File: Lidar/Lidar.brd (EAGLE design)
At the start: 100 x 80 mm, 4 parts

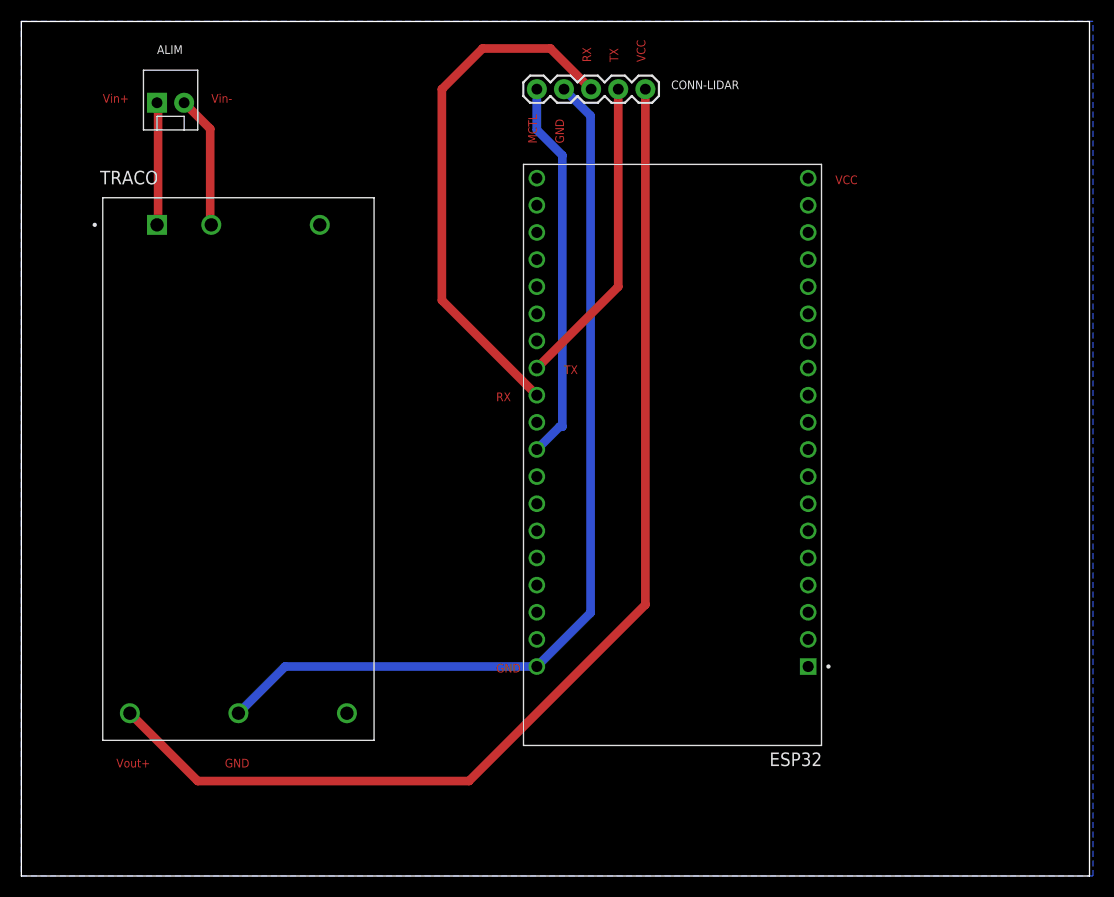
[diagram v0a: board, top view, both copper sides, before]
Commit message: re-route everything
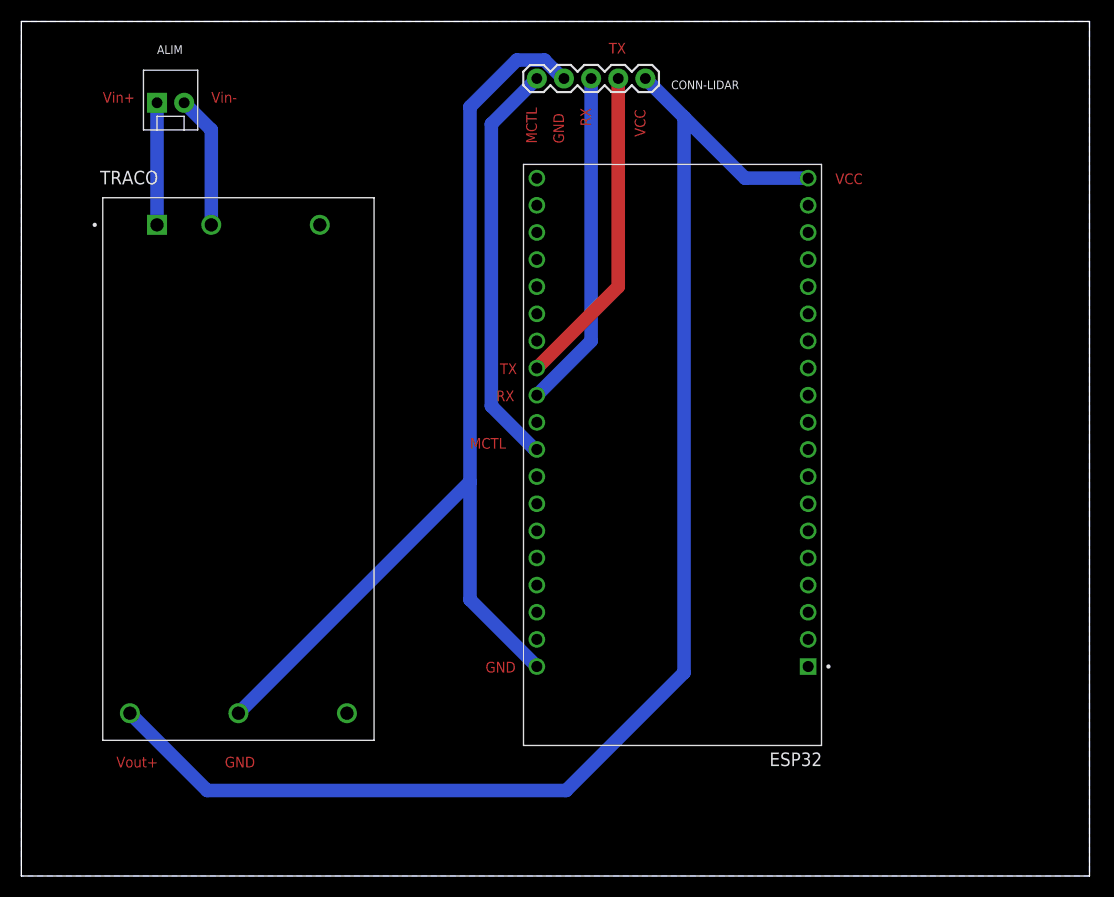
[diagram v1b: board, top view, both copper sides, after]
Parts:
- moved CONN-LIDAR 1.00 mm to (58.4, 74.7)
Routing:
- net VCC: track 106.2 -> 130.6 mm
- net RX: track 50.1 -> 31.8 mm
- net GND: track 87.2 -> 97.0 mm
- net MOTORCTL: track 35.9 -> 38.4 mm
- net TX: track 29.3 -> 30.3 mm, vias 1 -> 0
- added copper zone on layer 16, net GND
- removed copper zone on layer 16, net GNDPLATE
